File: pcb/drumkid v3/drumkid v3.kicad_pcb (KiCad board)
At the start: 2 copper layers, 90 x 120 mm, 61 parts, among them J1 Conn_01x04_Female, J5 Conn_01x05_Female, J6 Conn_01x04_Female, J7 Conn_01x06_Female, J8 Conn_01x05_Female, J9 AudioJack3_Ground_Switch, SW1 SW_SPDT, SW2 SW_Push, SW3 SW_Push, SW4 SW_Push, SW5 SW_Push, SW6 SW_Push, SW7 SW_Push, U2 ATmega328P-PU, U3 LM386, Y1 Crystal

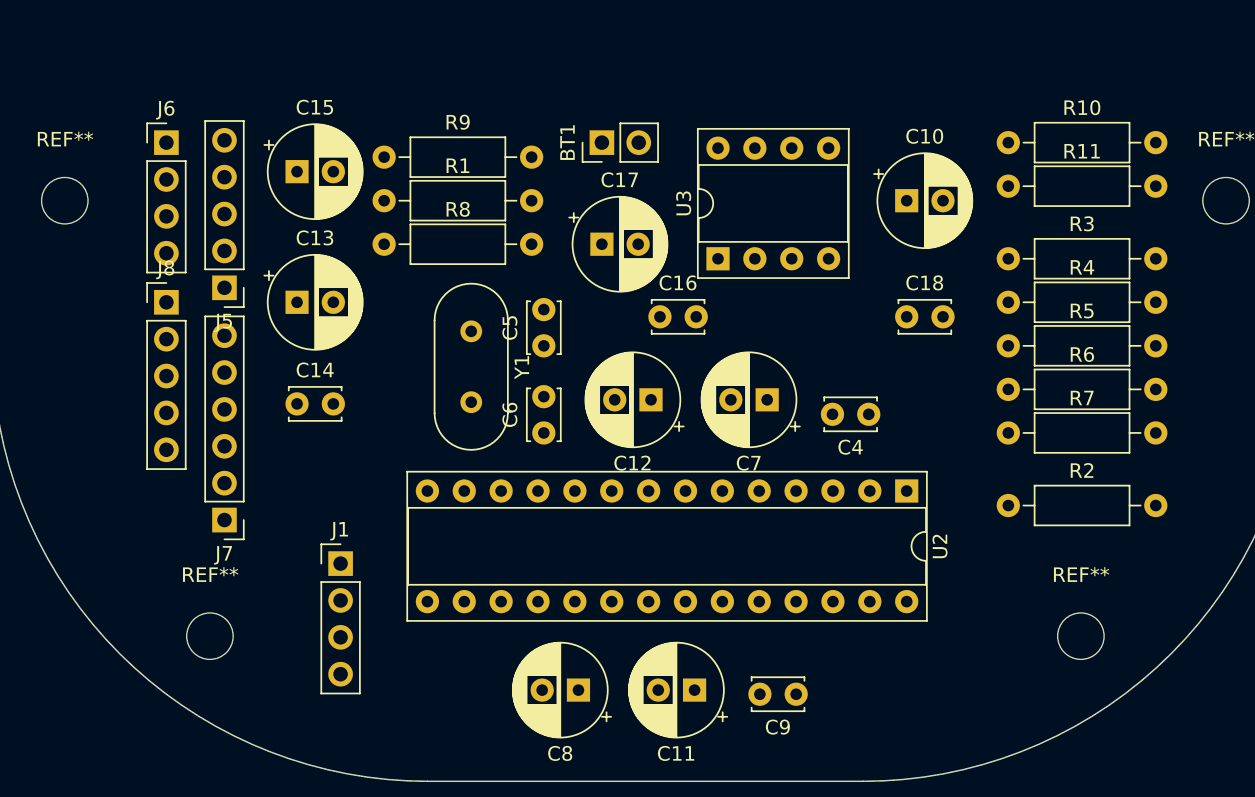
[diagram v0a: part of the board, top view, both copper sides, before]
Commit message: pcb layout looking nice (v3)
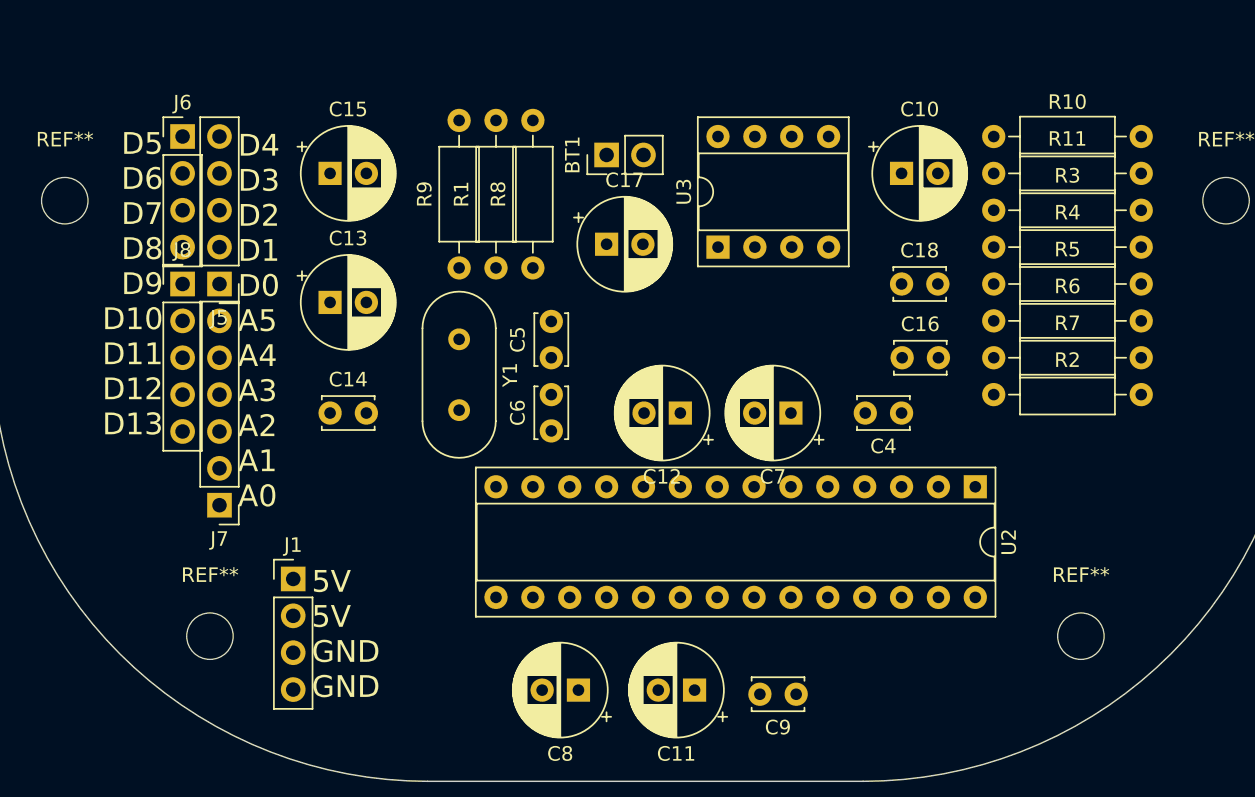
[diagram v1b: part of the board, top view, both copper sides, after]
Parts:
- moved C16 16.9 mm to (167.7, 130.8)
- moved R8 10.4 mm to (142.2, 124.6), turned to 90 degrees
- moved R9 9.22 mm to (137.2, 124.6), turned to 90 degrees
- moved R1 8.99 mm to (139.7, 124.6), turned to 90 degrees
- moved R2 7.71 mm to (174.0, 133.3)
- moved R7 5.28 mm to (174.0, 130.8)
- moved R6 4.83 mm to (174.0, 128.3)
- moved U2 4.74 mm to (172.7, 139.7)
- moved R5 4.38 mm to (174.0, 125.7)
- moved R4 3.93 mm to (174.0, 123.2)
- moved R3 3.49 mm to (174.0, 120.7)
- moved J1 3.43 mm to (125.7, 146.1)
- moved C14 2.36 mm to (128.3, 134.6)
- moved C18 2.29 mm to (167.6, 125.7)
- moved C15 2.28 mm to (128.3, 118.1)
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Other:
- board text added: "5V 5V GND GND"
- board text added: "D4 D3 D2 D1 D0 A5 A4 A3 A2 A1 A0"
- board text added: "D5 D6 D7 D8 D9 D10 D11 D12 D13"
